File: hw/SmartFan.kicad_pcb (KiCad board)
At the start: 2 copper layers, 102.5 x 68.5 mm, 25 parts, among them J1 DISPLAY, J2 Barrel_Jack, J3 JTAG_SWD, J4 Relay_Terminal, Q1 2N3904, Q2 2N3904, U1 hackaBLE_0.3, U2 L7805CV, U3 MCP23017_SP

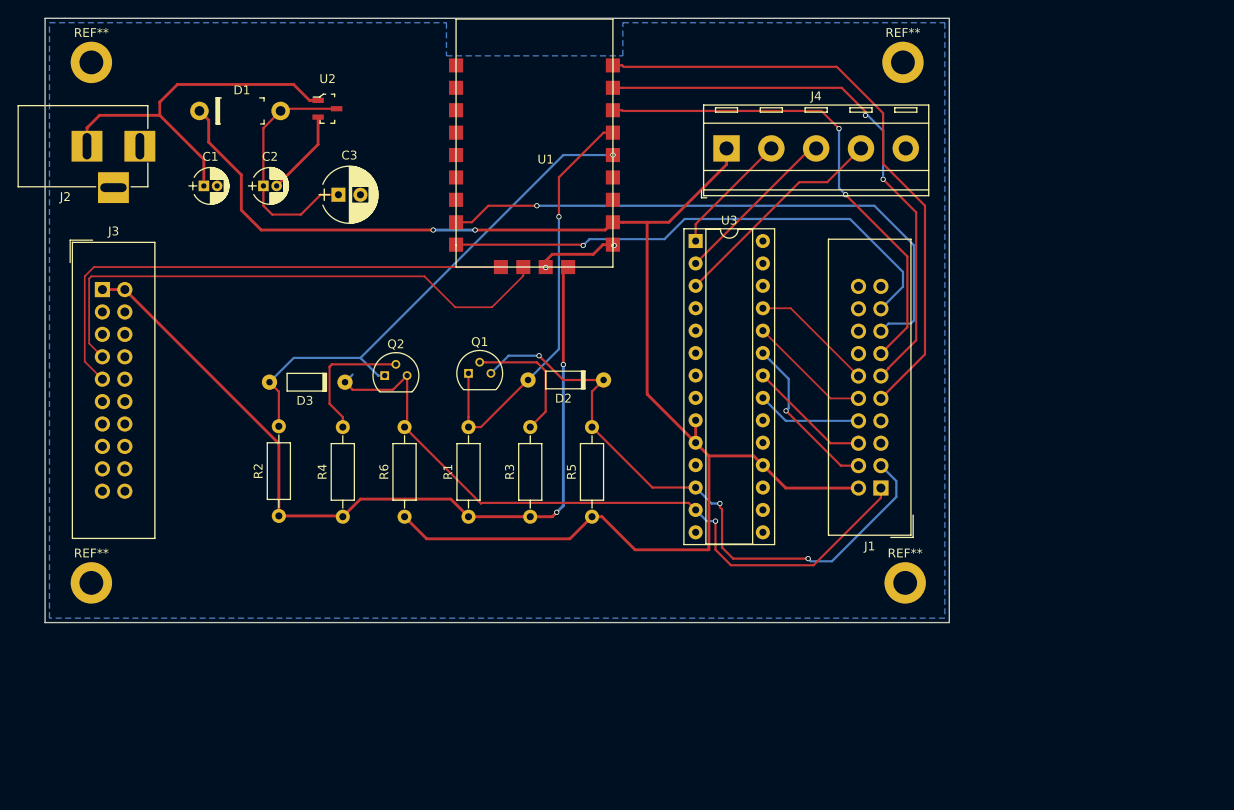
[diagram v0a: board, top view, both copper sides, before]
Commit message: Final v1 updates
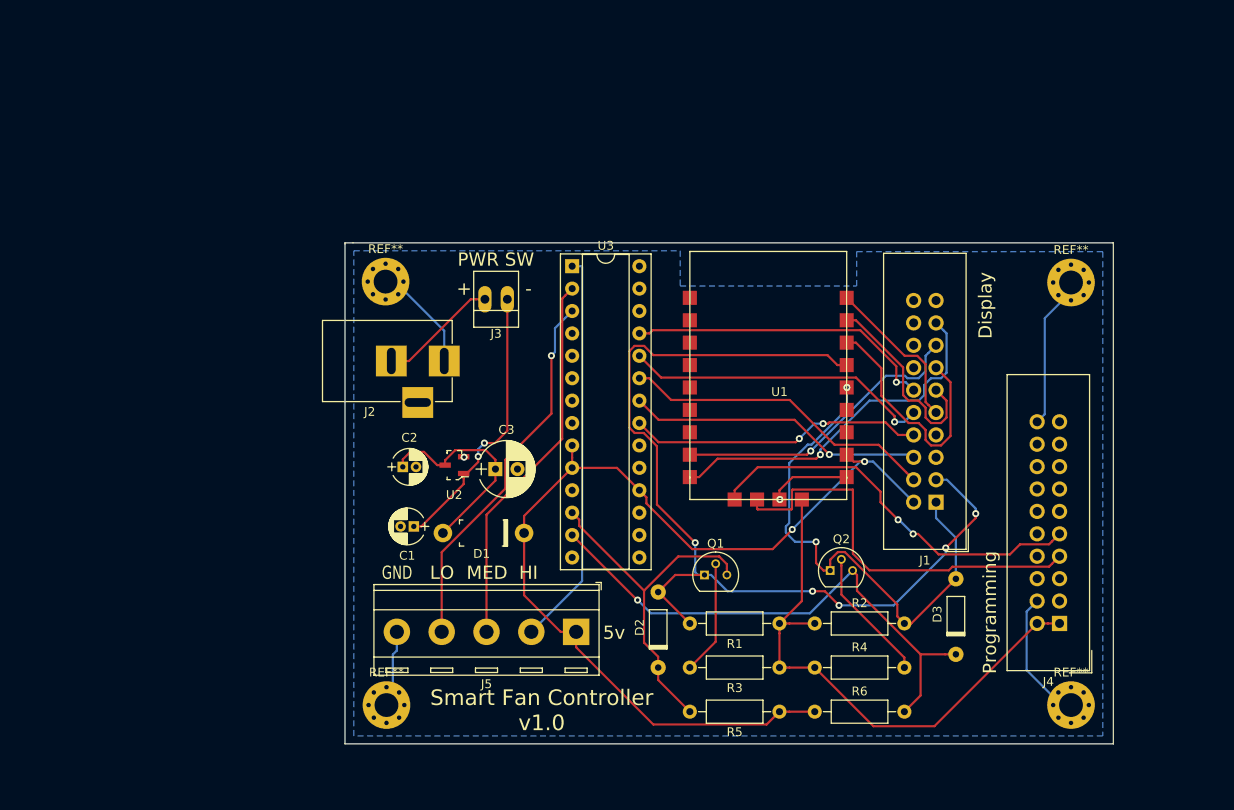
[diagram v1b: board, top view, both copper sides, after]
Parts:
- removed the REF** at (167.2, 39.8)
- removed the REF** at (167.5, 98.8)
- removed the REF** at (75.2, 39.8)
- removed the REF** at (75.2, 98.8)
- added J5: Relay_Terminal, TerminalBlock_RND:TerminalBlock_RND_205-00290_Pitch5.08mm, F.Cu at (130.2, 104.3)
- added REF**: MountingHole_2.7mm_M2.5_Pad_Via, Mounting_Holes:MountingHole_2.7mm_M2.5_Pad_Via, F.Cu at (108.6, 64.6)
- added REF**: MountingHole_2.7mm_M2.5_Pad_Via, Mounting_Holes:MountingHole_2.7mm_M2.5_Pad_Via, F.Cu at (186.3, 64.7)
- added REF**: MountingHole_2.7mm_M2.5_Pad_Via, Mounting_Holes:MountingHole_2.7mm_M2.5_Pad_Via, F.Cu at (186.3, 112.6)
- added REF**: MountingHole_2.7mm_M2.5_Pad_Via, Mounting_Holes:MountingHole_2.7mm_M2.5_Pad_Via, F.Cu at (108.7, 112.6)
- D1: footprint digikey-footprints:DO-41 -> Digikey:DO-41
- D2, D3: footprint digikey-footprints:DO-35 -> Digikey:DO-35
- J3: value JTAG_SWD -> PWR_SW; footprint Connectors_IDC:IDC-Header_2x10_Pitch2.54mm_Straight -> Connectors:PINHEAD1-2
- J4: value Relay_Terminal -> JTAG_SWD; footprint TerminalBlock_RND:TerminalBlock_RND_205-00290_Pitch5.08mm -> Connectors_IDC:IDC-Header_2x10_Pitch2.54mm_Straight
- U2: footprint digikey-footprints:SOT-23-3 -> Digikey:SOT-23-3
- moved D3 75.8 mm to (173.2, 106.8), turned to 90 degrees
- moved J4 65.8 mm to (185.0, 103.3), turned to 180 degrees
- moved R2 62.0 mm to (157.2, 103.3), turned to 0 degrees
- moved D1 60.4 mm to (124.3, 93.1), turned to 180 degrees
- moved R4 56.2 mm to (157.2, 108.3), turned to 0 degrees
- moved Q2 55.1 mm to (159.0, 97.3)
- moved R6 51.5 mm to (157.2, 113.3), turned to 0 degrees
- moved J3 45.9 mm to (122.4, 66.6), turned to 180 degrees
- moved C1 45.3 mm to (111.8, 92.3), turned to 180 degrees
- moved U2 42.9 mm to (116.4, 85.4), turned to 180 degrees
- moved J2 42.2 mm to (115.2, 73.6)
- moved U1 37.4 mm to (153.2, 76.6)
- moved R1 37.3 mm to (153.2, 103.3), turned to 180 degrees
- moved C3 35.8 mm to (121.0, 85.8)
- moved C2 35.6 mm to (110.5, 85.6)
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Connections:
- C1 pad 1: +9V -> Net-(C1-Pad1)
- D2 pad A: Net-(D2-PadA) -> /SCL_3v3
- D3 pad A: Net-(D3-PadA) -> /SDA_3v3
- J1 pad 1: /SDA_5v -> /SDA_3v3
- J1 pad 3: /SCL_5v -> /SCL_3v3
- J3 pad 1: +3V3 -> Net-(C1-Pad1)
- J3 pad 2: +3V3 -> +9V
- J4 pad 1: +5V -> +3V3
- J4 pad 2: /HI_SPD_EN -> +3V3
- J4 pad 3: /MED_SPD_EN -> Net-(J4-Pad3)
- J4 pad 4: /LO_SPD_EN -> GND
- J4 pad 5: GND -> Net-(J4-Pad5)
- Q1 pad 1: Net-(D2-PadA) -> /SCL_3v3
- Q2 pad 1: Net-(D3-PadA) -> /SDA_3v3
- R1 pad 2: Net-(D2-PadA) -> /SCL_3v3
- R2 pad 2: Net-(D3-PadA) -> /SDA_3v3
- U1 pad 13: Net-(D2-PadA) -> /SCL_3v3
- U1 pad 14: Net-(D3-PadA) -> /SDA_3v3
- U2 pad 1: +9V -> Net-(C1-Pad1)
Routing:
- net /SCL_3v3: track 0.00 -> 109.7 mm, vias 0 -> 5
- net +5V: track 173.2 -> 111.2 mm
- net /SDA_3v3: track 0.00 -> 59.9 mm, vias 0 -> 2
- net Net-(D3-PadA): track 58.6 -> 0.00 mm, vias 1 -> 0
- net /ROT_ENC_A: track 69.2 -> 18.0 mm
- net Net-(D2-PadA): track 47.7 -> 0.00 mm, vias 1 -> 0
- net GND: track 18.9 -> 62.8 mm
- net /ROT_ENC_B: track 63.9 -> 22.5 mm, vias 2 -> 0
- net +3V3: track 97.2 -> 63.4 mm, vias 2 -> 0
- net /ROT_ENC_SW1: track 67.3 -> 34.3 mm, vias 4 -> 1
- net Net-(C1-Pad1): track 0.00 -> 31.5 mm, vias 0 -> 2
- net /HI_SPD_EN: track 14.1 -> 44.9 mm
- net /SCL_5v: track 71.5 -> 40.7 mm, vias 4 -> 0
- net +9V: track 42.0 -> 13.5 mm
- net /ROT_ENC_C: track 56.5 -> 28.0 mm, vias 2 -> 0
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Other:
- board size 102.5 x 68.5 mm -> 87.1 x 56.8 mm
- net class 120VAC removed
- net class Data removed
- net class Default: via_dia 0.6 -> 0.8
- net class PWR removed
- rule pad_to_mask_clearance: 0.2 -> 0
- board text added: "+"
- board text added: "-"
- board text added: "5v"
- board text added: "Display"
- board text added: "GND"
- board text added: "HI"
- board text added: "LO"
- board text added: "MED"
- board text added: "PWR SW"
- board text added: "Programming"
- board text added: "Smart Fan Controller v1.0"

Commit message: Hardware design updates
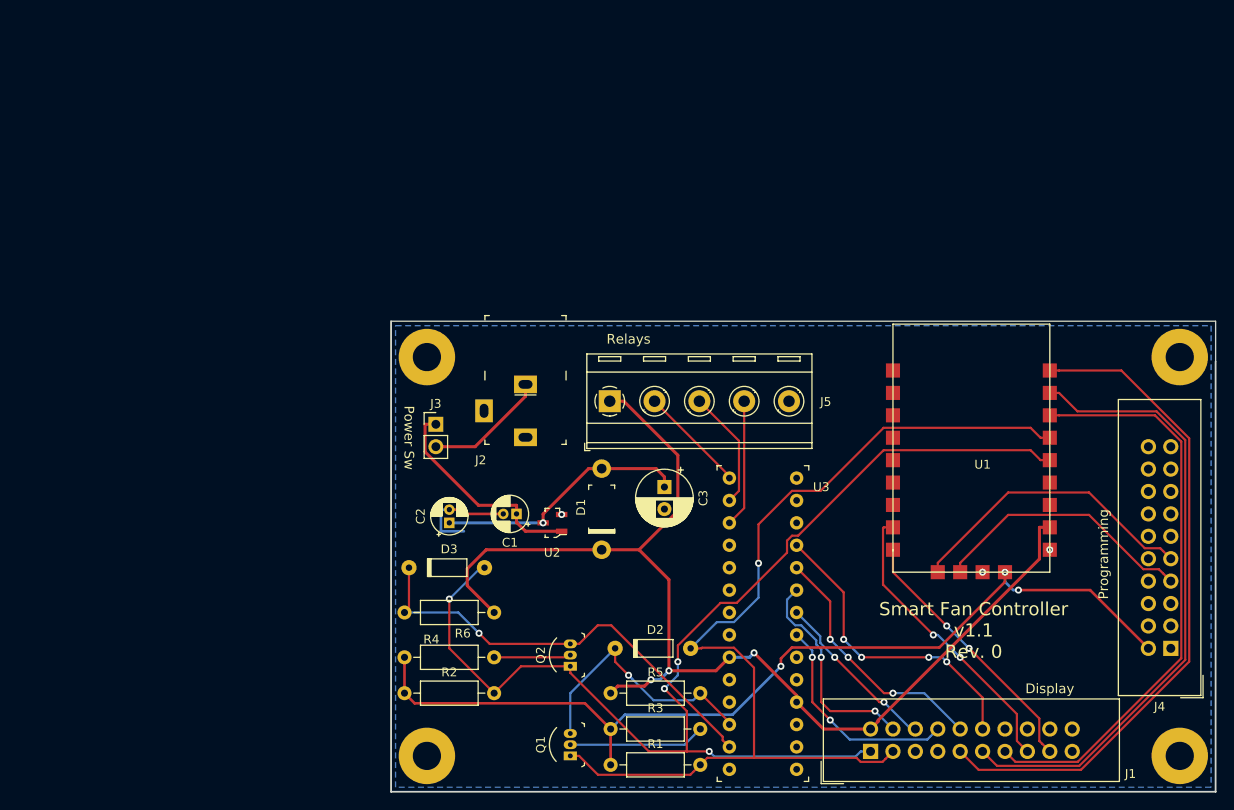
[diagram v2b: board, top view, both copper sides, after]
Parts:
- removed the REF** at (108.6, 64.6)
- removed the REF** at (186.3, 64.7)
- removed the REF** at (186.3, 112.6)
- removed the REF** at (108.7, 112.6)
- added REF**: MountingHole_3.2mm_M3_Pad, MountingHole:MountingHole_3.2mm_M3_Pad, F.Cu at (113.3, 118.4)
- added REF**: MountingHole_3.2mm_M3_Pad, MountingHole:MountingHole_3.2mm_M3_Pad, F.Cu at (113.3, 73.2)
- added REF**: MountingHole_3.2mm_M3_Pad, MountingHole:MountingHole_3.2mm_M3_Pad, F.Cu at (198.6, 118.4)
- added REF**: MountingHole_3.2mm_M3_Pad, MountingHole:MountingHole_3.2mm_M3_Pad, F.Cu at (198.6, 73.2)
- C1, C2: footprint Capacitors_THT:CP_Radial_D4.0mm_P1.50mm -> Capacitor_THT:CP_Radial_D4.0mm_P1.50mm
- C3: footprint Capacitors_THT:CP_Radial_D6.3mm_P2.50mm -> Capacitor_THT:CP_Radial_D6.3mm_P2.50mm
- D1: footprint Digikey:DO-41 -> digikey-footprints:DO-41
- D2, D3: footprint Digikey:DO-35 -> digikey-footprints:DO-35
- J1, J4: footprint Connectors_IDC:IDC-Header_2x10_Pitch2.54mm_Straight -> Connector_IDC:IDC-Header_2x10_P2.54mm_Vertical
- J2: value Barrel_Jack -> PJ-102A; footprint Connectors:BARREL_JACK -> digikey-footprints:Barrel_Jack_5.5mmODx2.1mmID_PJ-102A
- J3: footprint Connectors:PINHEAD1-2 -> Connector_PinHeader_2.54mm:PinHeader_1x02_P2.54mm_Vertical
- J5: footprint TerminalBlock_RND:TerminalBlock_RND_205-00290_Pitch5.08mm -> TerminalBlock_RND:TerminalBlock_RND_205-00290_1x05_P5.08mm_Horizontal
- Q1, Q2: footprint TO_SOT_Packages_THT:TO-92_Molded_Narrow -> digikey-footprints:TO-92-3
- R1, R2, R3, R4, R5, R6: footprint Resistors_THT:R_Axial_DIN0207_L6.3mm_D2.5mm_P10.16mm_Horizontal -> Resistor_THT:R_Axial_DIN0207_L6.3mm_D2.5mm_P10.16mm_Horizontal
- U2: footprint Digikey:SOT-23-3 -> digikey-footprints:SOT-23-3
- U3: footprint Housings_DIP:DIP-28_W7.62mm_Socket -> digikey-footprints:Socket_DIP-28_7.62mm_Conn
- moved D3 62.8 mm to (111.3, 97.0), turned to 0 degrees
- moved R2 47.2 mm to (110.7, 111.3)
- moved R4 46.5 mm to (110.7, 107.2)
- moved R6 38.0 mm to (120.9, 102.1), turned to 180 degrees
- moved Q2 31.4 mm to (129.5, 108.2), turned to 90 degrees
- moved U3 29.9 mm to (147.6, 86.9)
- moved J1 29.2 mm to (163.6, 117.9), turned to 90 degrees
- moved J5 26.4 mm to (134.0, 78.2), turned to 0 degrees
- moved Q1 25.5 mm to (129.5, 118.4), turned to 90 degrees
- moved R1 25.0 mm to (134.1, 119.4), turned to 0 degrees
- moved U1 24.5 mm to (176.3, 84.8)
- moved R3 20.4 mm to (134.1, 115.3), turned to 0 degrees
- moved C3 19.3 mm to (140.2, 87.9), turned to 270 degrees
- moved R5 19.3 mm to (134.1, 111.3), turned to 0 degrees
- moved J3 16.3 mm to (114.3, 80.8), turned to 0 degrees
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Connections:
- U3 pad 10: +5V -> GND
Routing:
- net /SDA_3v3: track 59.9 -> 133.4 mm, vias 2 -> 4
- net /ROT_ENC_A: track 18.0 -> 76.2 mm
- net GND: track 62.8 -> 12.2 mm, vias 2 -> 3
- net /ROT_ENC_B: track 22.5 -> 71.1 mm
- net +3V3: track 63.4 -> 106.9 mm, vias 0 -> 3
- net /ROT_ENC_C: track 28.0 -> 66.0 mm
- net /HI_SPD_EN: track 44.9 -> 12.2 mm
- net /MED_SPD_EN: track 42.9 -> 13.6 mm
- net /LO_SPD_EN: track 42.5 -> 14.5 mm, vias 1 -> 0
- net +5V: track 111.2 -> 131.8 mm, vias 2 -> 3
- net /SWDIO: track 46.3 -> 30.3 mm
- net /RGB_Y: track 33.8 -> 19.4 mm, vias 1 -> 2
- net /RGB_G: track 35.9 -> 24.5 mm, vias 0 -> 2
- net /SDA_5v: track 61.4 -> 50.4 mm
- net /ROT_ENC_SW2: track 41.1 -> 30.2 mm, vias 1 -> 2
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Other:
- board size 87.1 x 56.8 mm -> 93.5 x 53.3 mm
- net class 3v added: clearance 0.2, trace_width 0.3, via_dia 0.8, via_drill 0.4
- net class 5v added: clearance 0.2, trace_width 0.35, via_dia 0.8, via_drill 0.4
- net class 9v added: clearance 0.2, trace_width 0.35, via_dia 0.8, via_drill 0.4
- net class GND added: clearance 0.2, trace_width 0.3, via_dia 0.8, via_drill 0.4
- board text added: "Power Sw"
- board text added: "Relays"
- board text added: "Smart Fan Controller v1.1 Rev. 0"
- board text removed: "+"
- board text removed: "-"
- board text removed: "5v"
- board text removed: "GND"
- board text removed: "HI"
- board text removed: "LO"
- board text removed: "MED"
- board text removed: "PWR SW"
- board text removed: "Smart Fan Controller v1.0"
